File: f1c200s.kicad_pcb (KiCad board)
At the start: 4 copper layers, 100 x 100 mm, 44 parts, among them J1 Micro_SD_Card, J10 Conn_01x07, J2 USB_B_Micro, J3 Conn_01x03, J4 Conn_01x07, J5 Jumper, J6 Jumper, J7 Jumper, J8 Jumper, J9 Conn_01x01, Q1 2N7002, SW1 SW_Push, U1 F1C100s, U2 LDK130PU-R, U3 LDK130PU-R, U4 LDK130PU-R, Y1 XRCGB24M000F0G00R0

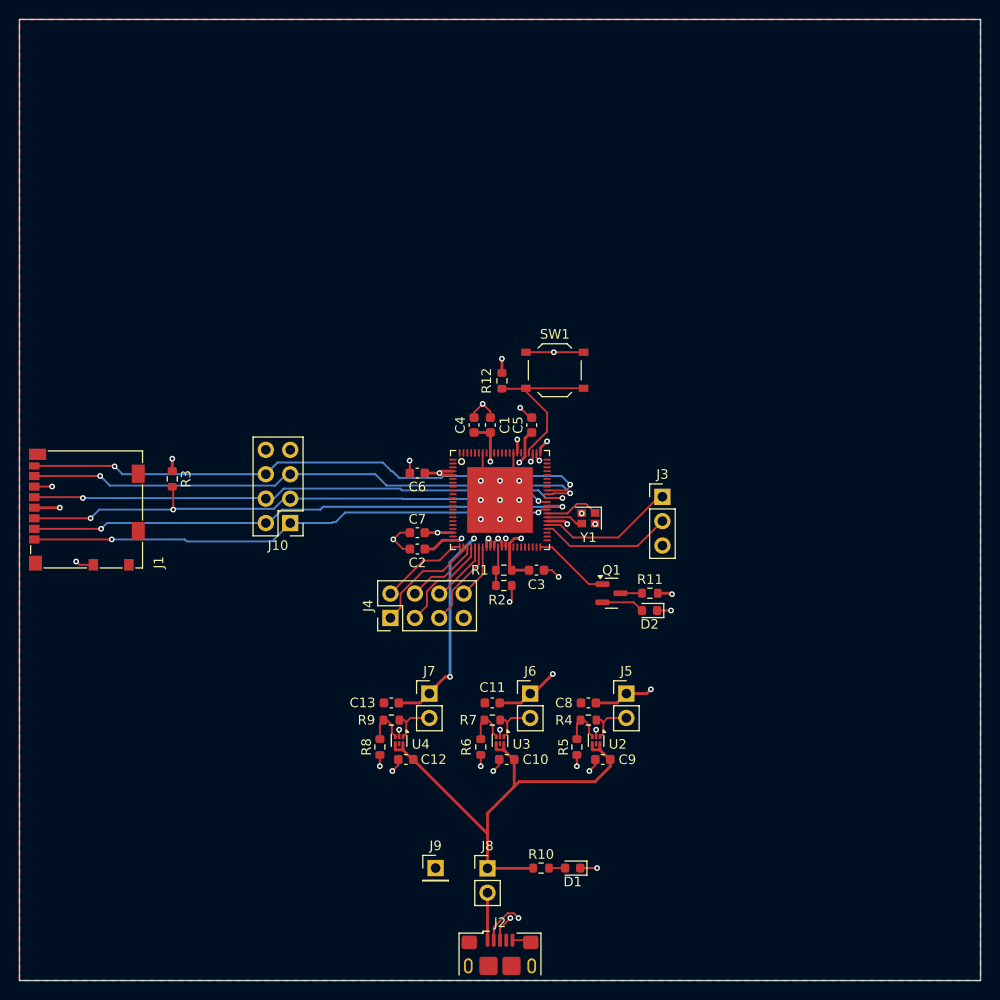
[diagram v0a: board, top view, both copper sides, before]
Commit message: Dev board V2
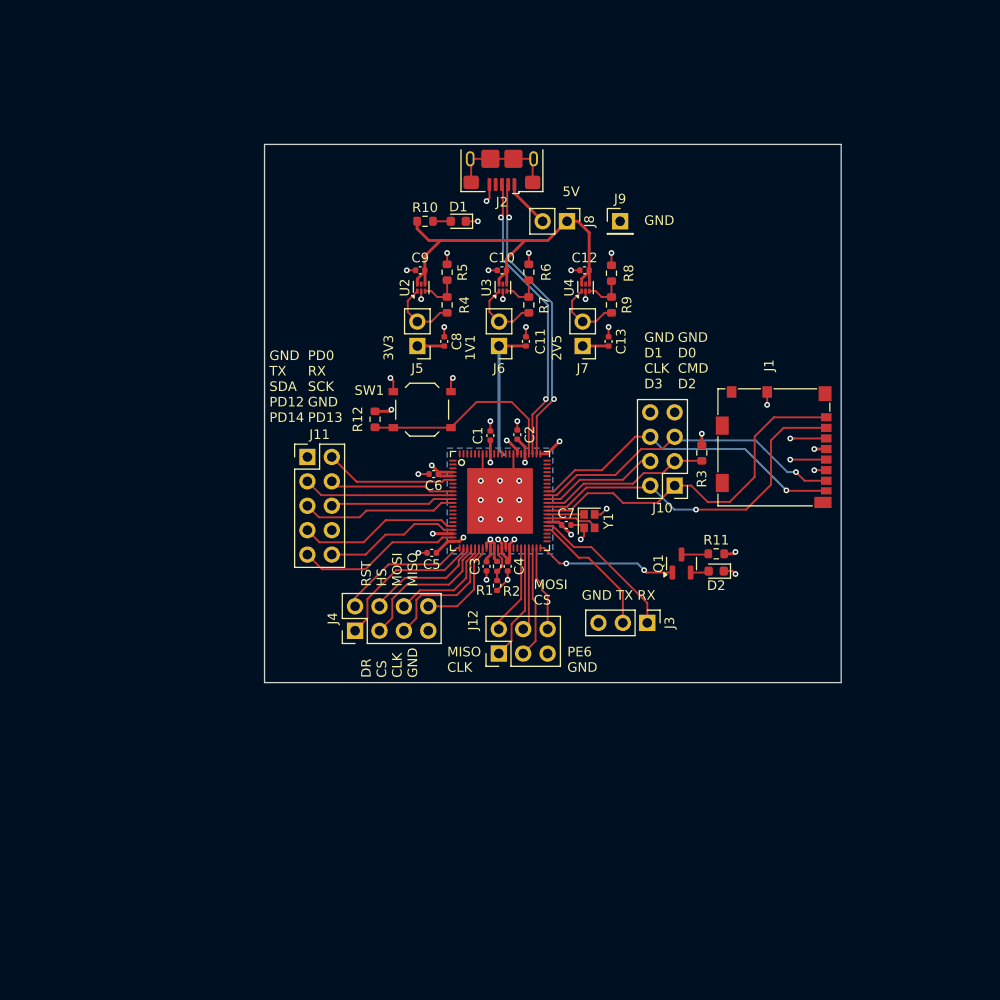
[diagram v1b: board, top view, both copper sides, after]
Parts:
- added J11: Conn_02x05_Odd_Even, Connector_PinHeader_2.54mm:PinHeader_2x05_P2.54mm_Vertical, F.Cu at (130.0, 95.5)
- added J12: Conn_02x03_Odd_Even, Connector_PinHeader_2.54mm:PinHeader_2x03_P2.54mm_Vertical, F.Cu at (149.9, 116.0)
- C1, C10, C11, C12, C13, C2, C3, C4, C5, C6, C7, C8, C9: footprint Capacitor_SMD:C_0603_1608Metric -> Capacitor_SMD:C_0402_1005Metric
- R1, R2: value 5.1K -> 4.7k; footprint Resistor_SMD:R_0603_1608Metric -> Resistor_SMD:R_0402_1005Metric
- moved J2 84.0 mm to (150.2, 64.5), turned to 180 degrees
- moved J1 71.8 mm to (178.5, 94.5), turned to -90 degrees
- moved J9 70.0 mm to (162.5, 71.0)
- moved R10 68.4 mm to (142.2, 71.0)
- moved D1 68.3 mm to (145.7, 71.0)
- moved J8 67.8 mm to (157.0, 71.0), turned to -90 degrees
- moved R3 55.2 mm to (171.0, 95.1)
- moved R8 54.9 mm to (161.6, 76.4), turned to 90 degrees
- moved C9 54.3 mm to (141.7, 76.1)
- moved C12 54.2 mm to (158.8, 76.1)
- moved R5 51.2 mm to (144.5, 76.3), turned to 90 degrees
- moved U4 50.9 mm to (158.9, 77.9), turned to 90 degrees
- moved C10 50.9 mm to (150.2, 76.1)
- moved U2 50.5 mm to (141.8, 77.9), turned to 90 degrees
- moved R6 49.7 mm to (153.0, 76.3), turned to 90 degrees
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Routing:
- net /D-: track 58.7 -> 31.0 mm
- net /SDC0_D1: track 60.5 -> 33.7 mm, vias 2 -> 1
- net /SDC0_D0: track 59.9 -> 33.5 mm, vias 2 -> 1
- net /D+: track 56.7 -> 30.8 mm
- net /SDC0_CLK: track 57.5 -> 31.8 mm, vias 2 -> 1
- net /SDC0_CMD: track 57.1 -> 34.7 mm, vias 3 -> 1
- net /SDC0_D3: track 57.6 -> 37.2 mm, vias 2 -> 1
- net /PD14: track 0.00 -> 17.1 mm
- net /SDC0_D2: track 54.8 -> 37.8 mm, vias 2 -> 0
- net /PD12: track 0.00 -> 16.9 mm
- net /I2C1_SDA: track 0.00 -> 16.3 mm
- net /UART1_TX: track 0.00 -> 15.7 mm
- net /PD13: track 0.00 -> 14.2 mm
- net /PD0: track 0.00 -> 13.8 mm
- net /UART1_RX: track 0.00 -> 13.0 mm
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- added copper zone on B.Cu, net +1V1
- removed copper zone on In2.Cu, net +1V1
- removed copper zone on F.Cu, net GND
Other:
- board size 100 x 100 mm -> 60 x 56 mm
- board text added: "1V1"
- board text added: "2V5"
- board text added: "3V3"
- board text added: "5V"
- board text added: "DR CS CLK GND"
- board text added: "GND"
- board text added: "GND D0 CMD D2"
- board text added: "GND D1 CLK D3"
- board text added: "GND TX RX"
- board text added: "GND TX SDA PD12 PD14"
- board text added: "MISO CLK"
- board text added: "MOSI CS"
- board text added: "PD0 RX SCK GND PD13"
- board text added: "PE6 GND"
- board text added: "RST HS MOSI MISO"
